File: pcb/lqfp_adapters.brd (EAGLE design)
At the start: 71.1 x 83.8 mm, 21 parts, among them IC1 STM32F405RGT, IC2 STM32F303CBT, IC3 STM32F051K4T

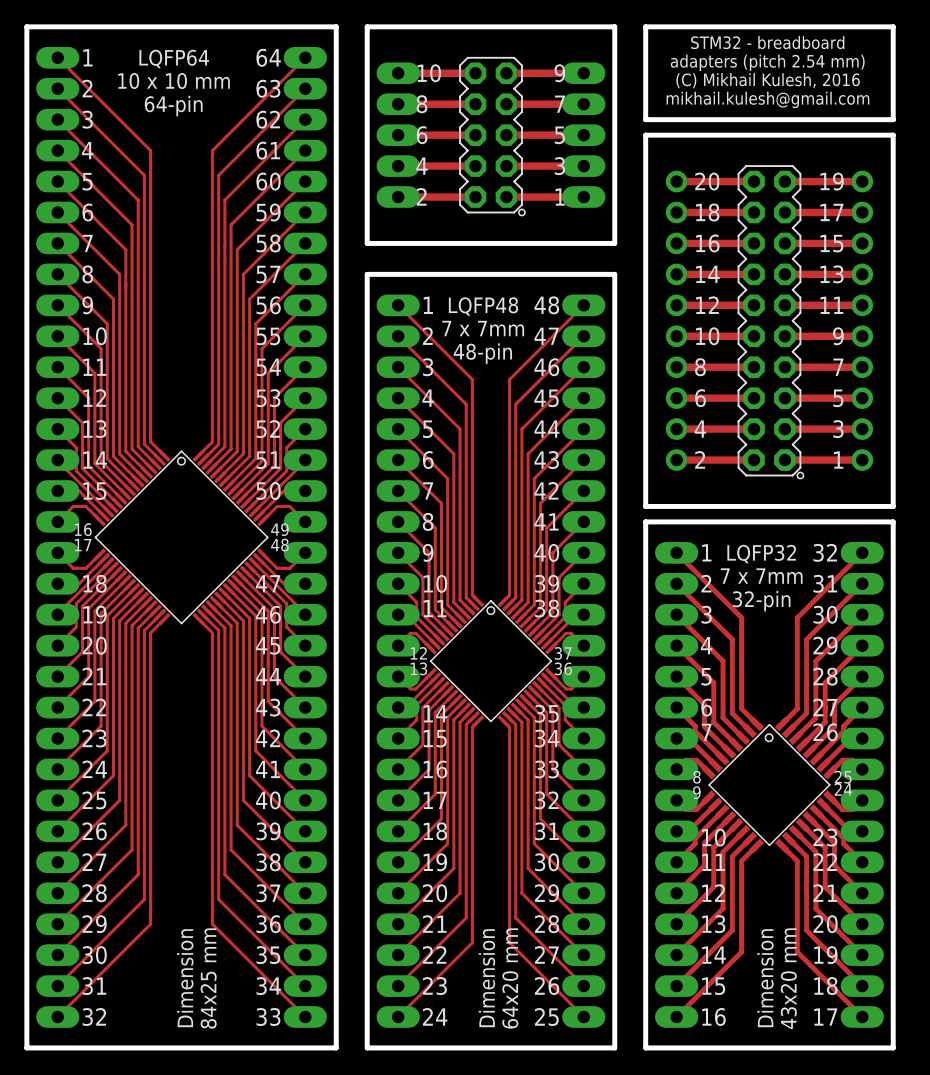
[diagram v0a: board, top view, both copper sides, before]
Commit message: Added version 2 of the boards
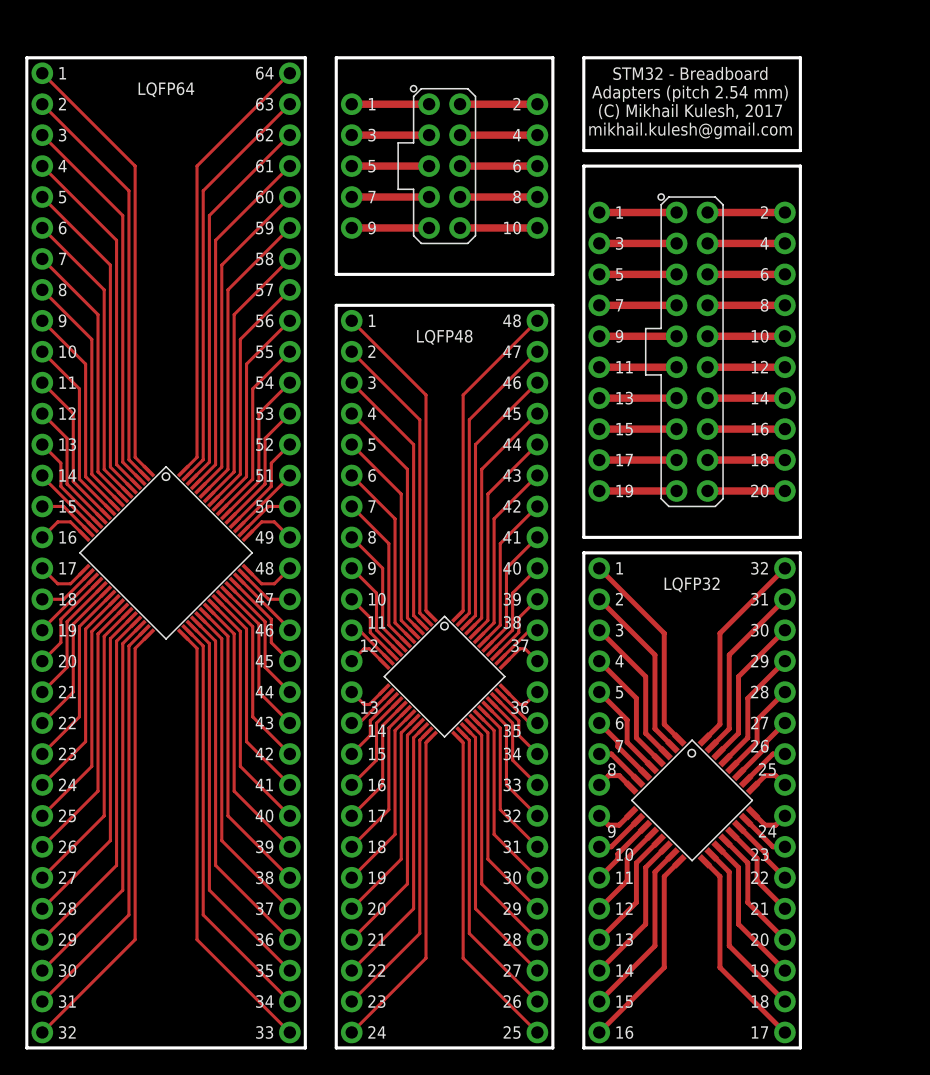
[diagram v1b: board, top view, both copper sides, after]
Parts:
- removed IC1: STM32F405RGT, stm32:LQFP64
- removed IC2: STM32F303CBT, stm32:LQFP48
- removed IC3: STM32F051K4T, stm32:LQFP32
- removed SV1, SV3: (no value), con-lstb:MA20-1
- removed SV10, SV11, SV12, SV9: (no value), con-lstb:MA08-1
- removed SV13: (no value), con-lstb:MA05-2
- removed SV14, SV15: (no value), con-lstb:MA05-1
- removed SV16: (no value), con-lstb:MA10-2
- removed SV17, SV18: (no value), con-lstb:MA10-1
- removed SV2, SV4, SV5, SV6, SV7, SV8: (no value), con-lstb:MA12-1
- added IC-A1: STM32F405RGT, stm32:LQFP64
- added IC-B1: STM32F303CBT, stm32:LQFP48
- added IC-E1: STM32F051K4T, stm32:LQFP32
- added SV-A1, SV-A4, SV-B1, SV-B2, SV-B3, SV-B4: (no value), MyComponents:MA12-1-NO-PL
- added SV-A2, SV-A3: (no value), MyComponents:MA20-1-NO-PL
- added SV-C1, SV-C3: (no value), MyComponents:MA05-1-NO-PL
- added SV-C2: (no value), MyComponents:MA05-2
- added SV-D1, SVD3: (no value), MyComponents:MA10-1-NO-PL
- added SV-D2: (no value), MyComponents:MA10-2
- added SV-E1, SV-E2, SV-E3, SV-E4: (no value), MyComponents:MA08-1-NO-PL
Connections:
- net A1: now also IC-A1.1, SV-A2.1; no longer IC1.1, SV1.1
- net A10: now also IC-A1.10, SV-A2.10; no longer IC1.10, SV1.10
- net A11: now also IC-A1.11, SV-A2.11; no longer IC1.11, SV1.11
- net A12: now also IC-A1.12, SV-A2.12; no longer IC1.12, SV1.12
- net A13: now also IC-A1.13, SV-A2.13; no longer IC1.13, SV1.13
- net A14: now also IC-A1.14, SV-A2.14; no longer IC1.14, SV1.14
- net A15: now also IC-A1.15, SV-A2.15; no longer IC1.15, SV1.15
- net A16: now also IC-A1.16, SV-A2.16; no longer IC1.16, SV1.16
- net A17: now also IC-A1.17, SV-A2.17; no longer IC1.17, SV1.17
- net A18: now also IC-A1.18, SV-A2.18; no longer IC1.18, SV1.18
- net A19: now also IC-A1.19, SV-A2.19; no longer IC1.19, SV1.19
- net A2: now also IC-A1.2, SV-A2.2; no longer IC1.2, SV1.2
- net A20: now also IC-A1.20, SV-A2.20; no longer IC1.20, SV1.20
- net A21: now also IC-A1.21, SV-A1.1; no longer IC1.21, SV2.1
- net A22: now also IC-A1.22, SV-A1.2; no longer IC1.22, SV2.2
- net A23: now also IC-A1.23, SV-A1.3; no longer IC1.23, SV2.3
- net A24: now also IC-A1.24, SV-A1.4; no longer IC1.24, SV2.4
- net A25: now also IC-A1.25, SV-A1.5; no longer IC1.25, SV2.5
- net A26: now also IC-A1.26, SV-A1.6; no longer IC1.26, SV2.6
- net A27: now also IC-A1.27, SV-A1.7; no longer IC1.27, SV2.7
- net A28: now also IC-A1.28, SV-A1.8; no longer IC1.28, SV2.8
- net A29: now also IC-A1.29, SV-A1.9; no longer IC1.29, SV2.9
- net A3: now also IC-A1.3, SV-A2.3; no longer IC1.3, SV1.3
- net A30: now also IC-A1.30, SV-A1.10; no longer IC1.30, SV2.10
- net A31: now also IC-A1.31, SV-A1.11; no longer IC1.31, SV2.11
- net A32: now also IC-A1.32, SV-A1.12; no longer IC1.32, SV2.12
- net A33: now also IC-A1.33, SV-A3.1; no longer IC1.33, SV3.1
- net A34: now also IC-A1.34, SV-A3.2; no longer IC1.34, SV3.2
- net A35: now also IC-A1.35, SV-A3.3; no longer IC1.35, SV3.3
- net A36: now also IC-A1.36, SV-A3.4; no longer IC1.36, SV3.4
- net A37: now also IC-A1.37, SV-A3.5; no longer IC1.37, SV3.5
- net A38: now also IC-A1.38, SV-A3.6; no longer IC1.38, SV3.6
- net A39: now also IC-A1.39, SV-A3.7; no longer IC1.39, SV3.7
- net A4: now also IC-A1.4, SV-A2.4; no longer IC1.4, SV1.4
- net A40: now also IC-A1.40, SV-A3.8; no longer IC1.40, SV3.8
- net A41: now also IC-A1.41, SV-A3.9; no longer IC1.41, SV3.9
- net A42: now also IC-A1.42, SV-A3.10; no longer IC1.42, SV3.10
- net A43: now also IC-A1.43, SV-A3.11; no longer IC1.43, SV3.11
- net A44: now also IC-A1.44, SV-A3.12; no longer IC1.44, SV3.12
- net A45: now also IC-A1.45, SV-A3.13; no longer IC1.45, SV3.13
- net A46: now also IC-A1.46, SV-A3.14; no longer IC1.46, SV3.14
- net A47: now also IC-A1.47, SV-A3.15; no longer IC1.47, SV3.15
- net A48: now also IC-A1.48, SV-A3.16; no longer IC1.48, SV3.16
- net A49: now also IC-A1.49, SV-A3.17; no longer IC1.49, SV3.17
- net A5: now also IC-A1.5, SV-A2.5; no longer IC1.5, SV1.5
- net A50: now also IC-A1.50, SV-A3.18; no longer IC1.50, SV3.18
- net A51: now also IC-A1.51, SV-A3.19; no longer IC1.51, SV3.19
- net A52: now also IC-A1.52, SV-A3.20; no longer IC1.52, SV3.20
- net A53: now also IC-A1.53, SV-A4.1; no longer IC1.53, SV4.1
- net A54: now also IC-A1.54, SV-A4.2; no longer IC1.54, SV4.2
- net A55: now also IC-A1.55, SV-A4.3; no longer IC1.55, SV4.3
- net A56: now also IC-A1.56, SV-A4.4; no longer IC1.56, SV4.4
- net A57: now also IC-A1.57, SV-A4.5; no longer IC1.57, SV4.5
- net A58: now also IC-A1.58, SV-A4.6; no longer IC1.58, SV4.6
- net A59: now also IC-A1.59, SV-A4.7; no longer IC1.59, SV4.7
- net A6: now also IC-A1.6, SV-A2.6; no longer IC1.6, SV1.6
- net A60: now also IC-A1.60, SV-A4.8; no longer IC1.60, SV4.8
- net A61: now also IC-A1.61, SV-A4.9; no longer IC1.61, SV4.9
- net A62: now also IC-A1.62, SV-A4.10; no longer IC1.62, SV4.10
- net A63: now also IC-A1.63, SV-A4.11; no longer IC1.63, SV4.11
- net A64: now also IC-A1.64, SV-A4.12; no longer IC1.64, SV4.12
- net A7: now also IC-A1.7, SV-A2.7; no longer IC1.7, SV1.7
- net A8: now also IC-A1.8, SV-A2.8; no longer IC1.8, SV1.8
- net A9: now also IC-A1.9, SV-A2.9; no longer IC1.9, SV1.9
- net B1: now also IC-B1.1, SV-B2.1; no longer IC2.1, SV5.1
- net B10: now also IC-B1.10, SV-B2.10; no longer IC2.10, SV5.10
- net B11: now also IC-B1.11, SV-B2.11; no longer IC2.11, SV5.11
- net B12: now also IC-B1.12, SV-B2.12; no longer IC2.12, SV5.12
- net B13: now also IC-B1.13, SV-B1.1; no longer IC2.13, SV6.1
- net B14: now also IC-B1.14, SV-B1.2; no longer IC2.14, SV6.2
- net B15: now also IC-B1.15, SV-B1.3; no longer IC2.15, SV6.3
- net B16: now also IC-B1.16, SV-B1.4; no longer IC2.16, SV6.4
- net B17: now also IC-B1.17, SV-B1.5; no longer IC2.17, SV6.5
- net B18: now also IC-B1.18, SV-B1.6; no longer IC2.18, SV6.6
- net B19: now also IC-B1.19, SV-B1.7; no longer IC2.19, SV6.7
- net B2: now also IC-B1.2, SV-B2.2; no longer IC2.2, SV5.2
- net B20: now also IC-B1.20, SV-B1.8; no longer IC2.20, SV6.8
- net B21: now also IC-B1.21, SV-B1.9; no longer IC2.21, SV6.9
- net B22: now also IC-B1.22, SV-B1.10; no longer IC2.22, SV6.10
- net B23: now also IC-B1.23, SV-B1.11; no longer IC2.23, SV6.11
- net B24: now also IC-B1.24, SV-B1.12; no longer IC2.24, SV6.12
- net B25: now also IC-B1.25, SV-B3.1; no longer IC2.25, SV7.1
- net B26: now also IC-B1.26, SV-B3.2; no longer IC2.26, SV7.2
- net B27: now also IC-B1.27, SV-B3.3; no longer IC2.27, SV7.3
- net B28: now also IC-B1.28, SV-B3.4; no longer IC2.28, SV7.4
- net B29: now also IC-B1.29, SV-B3.5; no longer IC2.29, SV7.5
- net B3: now also IC-B1.3, SV-B2.3; no longer IC2.3, SV5.3
- net B30: now also IC-B1.30, SV-B3.6; no longer IC2.30, SV7.6
- net B31: now also IC-B1.31, SV-B3.7; no longer IC2.31, SV7.7
- net B32: now also IC-B1.32, SV-B3.8; no longer IC2.32, SV7.8
- net B33: now also IC-B1.33, SV-B3.9; no longer IC2.33, SV7.9
- net B34: now also IC-B1.34, SV-B3.10; no longer IC2.34, SV7.10
- net B35: now also IC-B1.35, SV-B3.11; no longer IC2.35, SV7.11
- net B36: now also IC-B1.36, SV-B3.12; no longer IC2.36, SV7.12
- net B37: now also IC-B1.37, SV-B4.1; no longer IC2.37, SV8.1
- net B38: now also IC-B1.38, SV-B4.2; no longer IC2.38, SV8.2
- net B39: now also IC-B1.39, SV-B4.3; no longer IC2.39, SV8.3
- net B4: now also IC-B1.4, SV-B2.4; no longer IC2.4, SV5.4
- net B40: now also IC-B1.40, SV-B4.4; no longer IC2.40, SV8.4
- net B41: now also IC-B1.41, SV-B4.5; no longer IC2.41, SV8.5
- net B42: now also IC-B1.42, SV-B4.6; no longer IC2.42, SV8.6
- net B43: now also IC-B1.43, SV-B4.7; no longer IC2.43, SV8.7
- net B44: now also IC-B1.44, SV-B4.8; no longer IC2.44, SV8.8
- net B45: now also IC-B1.45, SV-B4.9; no longer IC2.45, SV8.9
- net B46: now also IC-B1.46, SV-B4.10; no longer IC2.46, SV8.10
- net B47: now also IC-B1.47, SV-B4.11; no longer IC2.47, SV8.11
- net B48: now also IC-B1.48, SV-B4.12; no longer IC2.48, SV8.12
- net B5: now also IC-B1.5, SV-B2.5; no longer IC2.5, SV5.5
- net B6: now also IC-B1.6, SV-B2.6; no longer IC2.6, SV5.6
- net B7: now also IC-B1.7, SV-B2.7; no longer IC2.7, SV5.7
- net B8: now also IC-B1.8, SV-B2.8; no longer IC2.8, SV5.8
- net B9: now also IC-B1.9, SV-B2.9; no longer IC2.9, SV5.9
- net E1: now also IC-E1.1, SV-E2.1; no longer IC3.1, SV9.1
- net E10: now also IC-E1.10, SV-E1.2; no longer IC3.10, SV10.2
- net E11: now also IC-E1.11, SV-E1.3; no longer IC3.11, SV10.3
- net E12: now also IC-E1.12, SV-E1.4; no longer IC3.12, SV10.4
- net E13: now also IC-E1.13, SV-E1.5; no longer IC3.13, SV10.5
- net E14: now also IC-E1.14, SV-E1.6; no longer IC3.14, SV10.6
- net E15: now also IC-E1.15, SV-E1.7; no longer IC3.15, SV10.7
- net E16: now also IC-E1.16, SV-E1.8; no longer IC3.16, SV10.8
- net E17: now also IC-E1.17, SV-E3.1; no longer IC3.17, SV11.1
- net E18: now also IC-E1.18, SV-E3.2; no longer IC3.18, SV11.2
- net E19: now also IC-E1.19, SV-E3.3; no longer IC3.19, SV11.3
- net E2: now also IC-E1.2, SV-E2.2; no longer IC3.2, SV9.2
- net E20: now also IC-E1.20, SV-E3.4; no longer IC3.20, SV11.4
- net E21: now also IC-E1.21, SV-E3.5; no longer IC3.21, SV11.5
- net E22: now also IC-E1.22, SV-E3.6; no longer IC3.22, SV11.6
- net E23: now also IC-E1.23, SV-E3.7; no longer IC3.23, SV11.7
- net E24: now also IC-E1.24, SV-E3.8; no longer IC3.24, SV11.8
- net E25: now also IC-E1.25, SV-E4.1; no longer IC3.25, SV12.1
- net E26: now also IC-E1.26, SV-E4.2; no longer IC3.26, SV12.2
- net E27: now also IC-E1.27, SV-E4.3; no longer IC3.27, SV12.3
- net E28: now also IC-E1.28, SV-E4.4; no longer IC3.28, SV12.4
- net E29: now also IC-E1.29, SV-E4.5; no longer IC3.29, SV12.5
- net E3: now also IC-E1.3, SV-E2.3; no longer IC3.3, SV9.3
- net E30: now also IC-E1.30, SV-E4.6; no longer IC3.30, SV12.6
- net E31: now also IC-E1.31, SV-E4.7; no longer IC3.31, SV12.7
- net E32: now also IC-E1.32, SV-E4.8; no longer IC3.32, SV12.8
- net E4: now also IC-E1.4, SV-E2.4; no longer IC3.4, SV9.4
- net E5: now also IC-E1.5, SV-E2.5; no longer IC3.5, SV9.5
- net E6: now also IC-E1.6, SV-E2.6; no longer IC3.6, SV9.6
- net E7: now also IC-E1.7, SV-E2.7; no longer IC3.7, SV9.7
- net E8: now also IC-E1.8, SV-E2.8; no longer IC3.8, SV9.8
- net E9: now also IC-E1.9, SV-E1.1; no longer IC3.9, SV10.1
- net N$1: now also SV-C2.1, SV-C3.1; no longer SV13.1, SV15.1
- net N$10: now also SV-C1.5, SV-C2.10; no longer SV13.10, SV14.5
- net N$11: now also SV-D2.1, SVD3.1; no longer SV16.1, SV18.1
- net N$13: now also SV-D2.3, SVD3.2; no longer SV16.3, SV18.2
- net N$14: now also SV-D2.5, SVD3.3; no longer SV16.5, SV18.3
- net N$17: now also SV-D2.7, SVD3.4; no longer SV16.7, SV18.4
- net N$2: now also SV-C2.3, SV-C3.2; no longer SV13.3, SV15.2
- net N$22: now also SV-D2.9, SVD3.5; no longer SV16.9, SV18.5
- net N$23: now also SV-D2.11, SVD3.6; no longer SV16.11, SV18.6
- net N$24: now also SV-D2.13, SVD3.7; no longer SV16.13, SV18.7
- net N$25: now also SV-D2.15, SVD3.8; no longer SV16.15, SV18.8
- net N$26: now also SV-D2.17, SVD3.9; no longer SV16.17, SV18.9
- net N$27: now also SV-D2.19, SVD3.10; no longer SV16.19, SV18.10
- net N$28: now also SV-D1.10, SV-D2.20; no longer SV16.20, SV17.10
- net N$29: now also SV-D1.9, SV-D2.18; no longer SV16.18, SV17.9
- net N$3: now also SV-C2.5, SV-C3.3; no longer SV13.5, SV15.3
- net N$31: now also SV-D1.8, SV-D2.16; no longer SV16.16, SV17.8
- net N$32: now also SV-D1.7, SV-D2.14; no longer SV16.14, SV17.7
- net N$33: now also SV-D1.6, SV-D2.12; no longer SV16.12, SV17.6
- net N$34: now also SV-D1.5, SV-D2.10; no longer SV16.10, SV17.5
- net N$35: now also SV-D1.4, SV-D2.8; no longer SV16.8, SV17.4
- net N$36: now also SV-D1.3, SV-D2.6; no longer SV16.6, SV17.3
- net N$37: now also SV-D1.2, SV-D2.4; no longer SV16.4, SV17.2
- net N$38: now also SV-D1.1, SV-D2.2; no longer SV16.2, SV17.1
- net N$4: now also SV-C2.7, SV-C3.4; no longer SV13.7, SV15.4
- net N$5: now also SV-C2.9, SV-C3.5; no longer SV13.9, SV15.5
- net N$6: now also SV-C1.1, SV-C2.2; no longer SV13.2, SV14.1
- net N$7: now also SV-C1.2, SV-C2.4; no longer SV13.4, SV14.2
- net N$8: now also SV-C1.3, SV-C2.6; no longer SV13.6, SV14.3
- net N$9: now also SV-C1.4, SV-C2.8; no longer SV13.8, SV14.4
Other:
- board size 71.1 x 83.8 mm -> 63.5 x 81.3 mm
- board text added: "LQFP32"
- board text added: "LQFP48"
- board text added: "LQFP64"
- board text added: "STM32 - Breadboard Adapters (pitch 2.54 mm) (C) Mikhail Kulesh, 2017 mikhail.kulesh@gmail.com"
- board text removed: "Dimension 43x20 mm"
- board text removed: "Dimension 64x20 mm"
- board text removed: "Dimension 84x25 mm"
- board text removed: "LQFP32 7 x 7mm 32-pin"
- board text removed: "LQFP48 7 x 7mm 48-pin"
- board text removed: "LQFP64 10 x 10 mm 64-pin"
- board text removed: "STM32 - breadboard adapters (pitch 2.54 mm) (C) Mikhail Kulesh, 2016 mikhail.kulesh@gmail.com"
